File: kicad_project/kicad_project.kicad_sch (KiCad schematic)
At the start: 30 parts, among them J1 USB_C_Receptacle_USB2.0_16P, Q2 DMG2302U, SW1 SW_Push, U1 STM32F031F6Px, U2 MCP73831-2-MC, U3 MCP4011-xxxxMS, U4 FT232RL, U5 LMZM23601

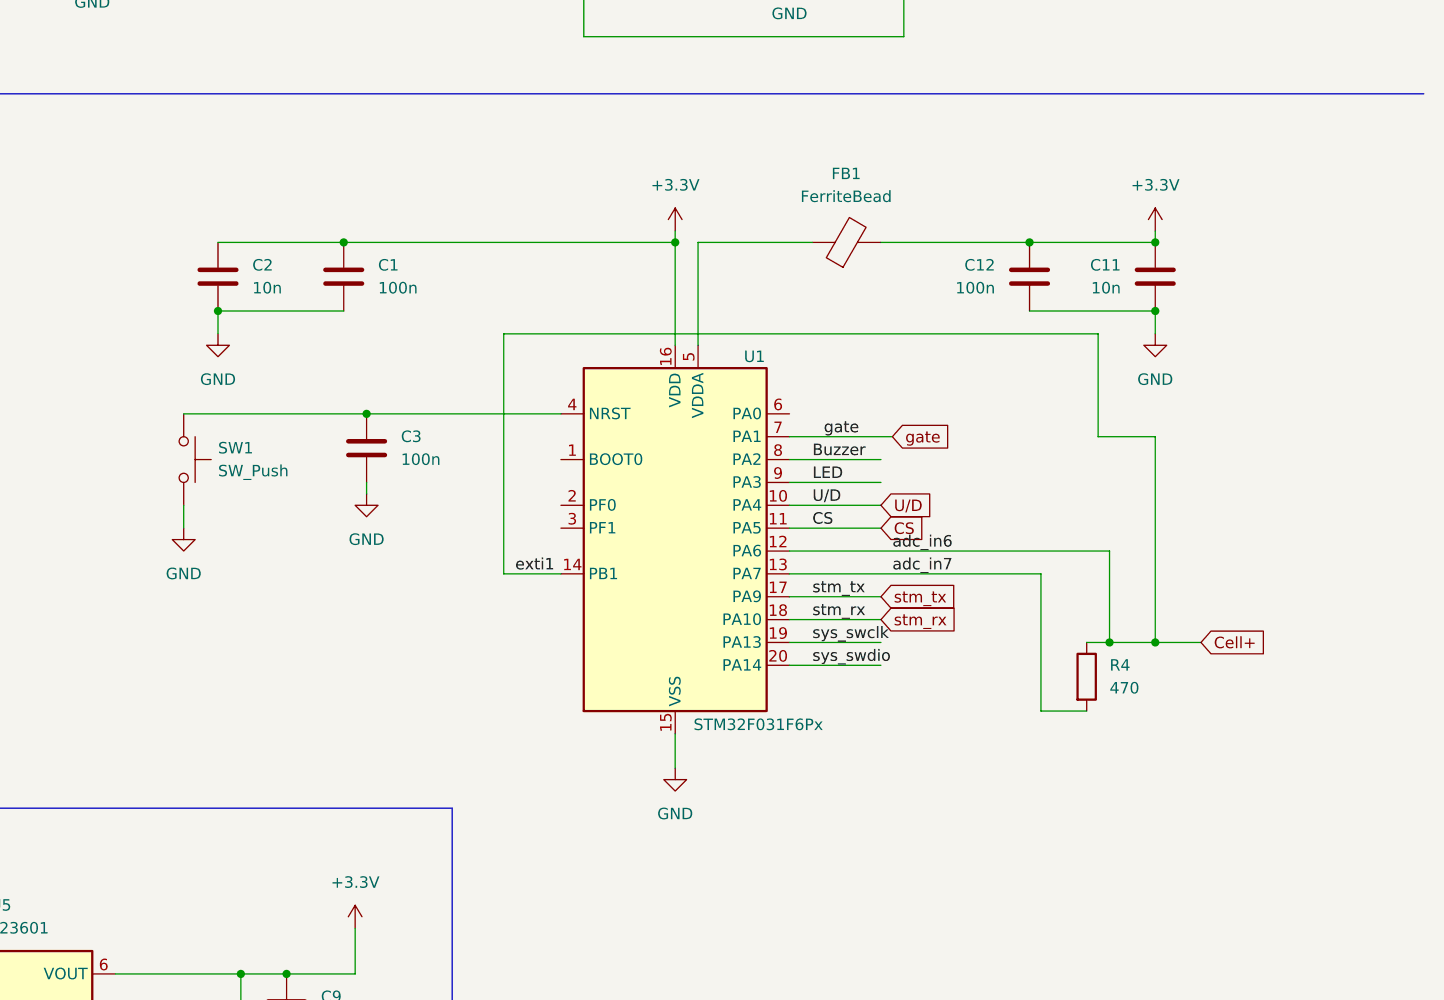
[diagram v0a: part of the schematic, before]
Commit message: edit done
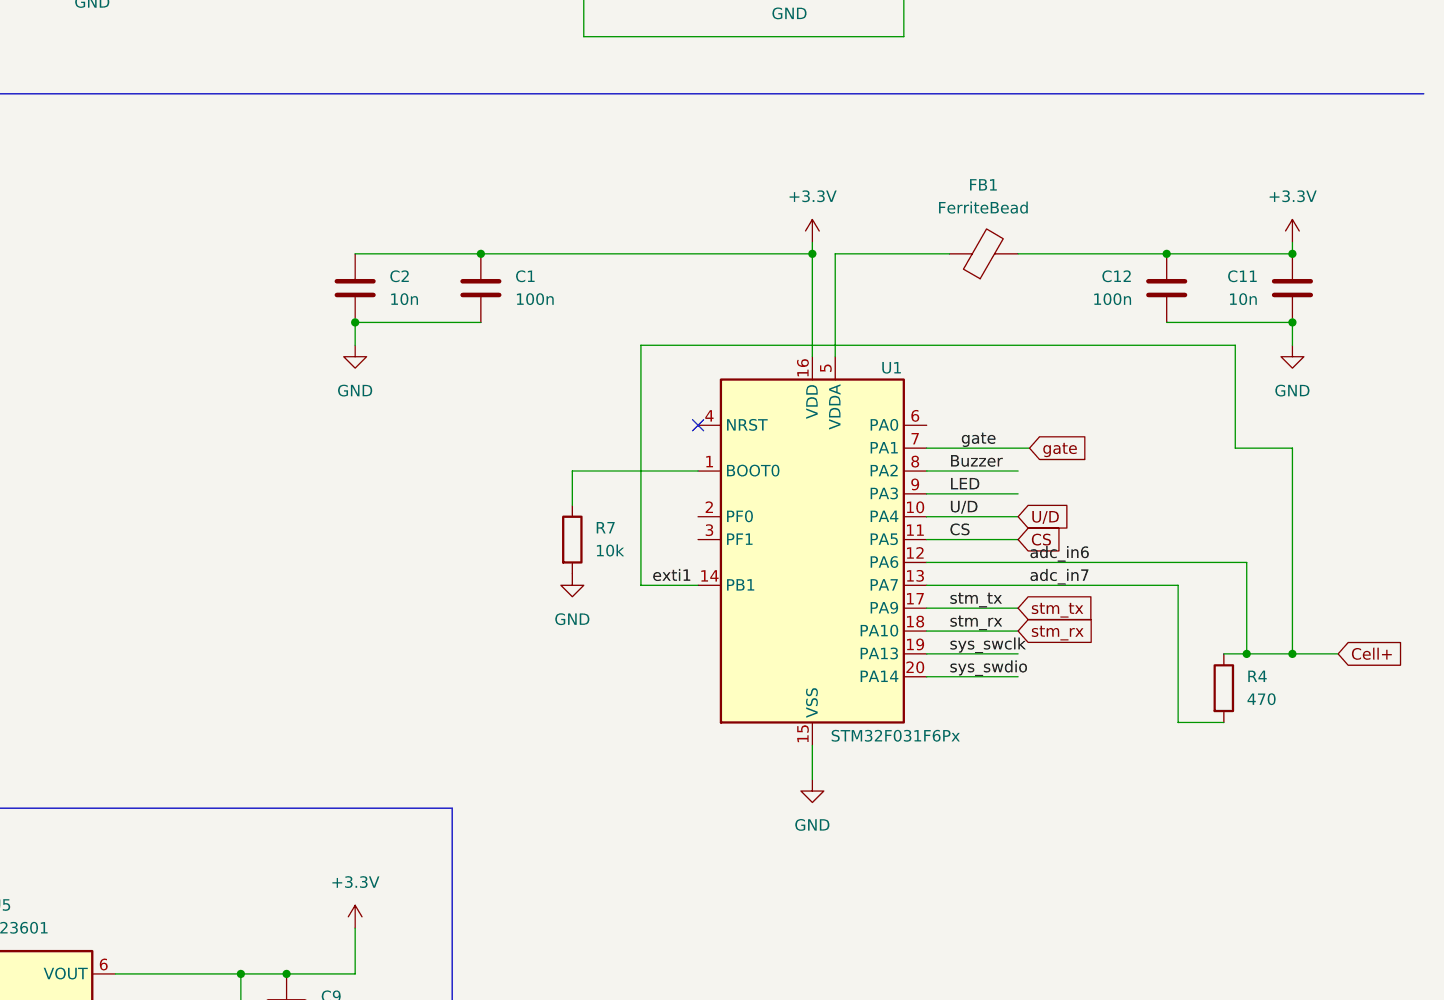
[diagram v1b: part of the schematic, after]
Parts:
- removed C3: 100n, symbol Device:C
- removed SW1: SW_Push, symbol Switch:SW_Push
- added R7: 10k, symbol Device:R
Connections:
- net GND: now also R7.2
- net at U1.1 (BOOT0): now also R7.1
- no-connect marks 16 -> 17
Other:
- moved on the sheet: C1, C11, C12, C2, FB1, R4, U1
